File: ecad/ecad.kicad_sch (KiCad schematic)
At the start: 0 parts

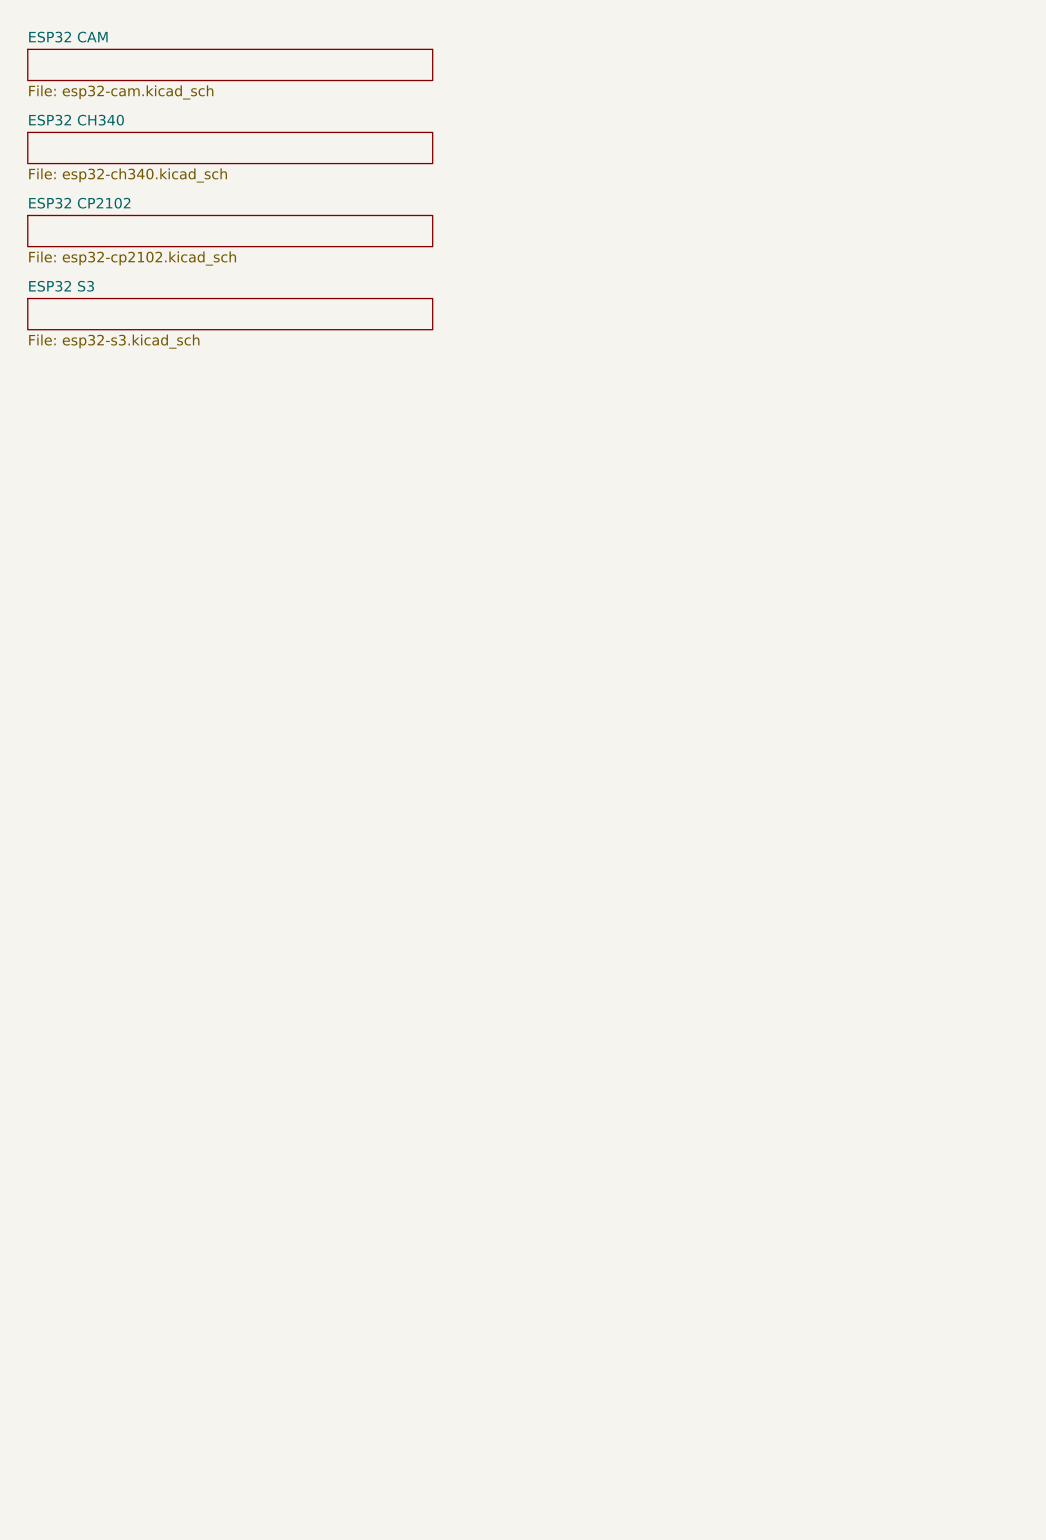
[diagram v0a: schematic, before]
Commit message: feat (ecad): update KiCad project
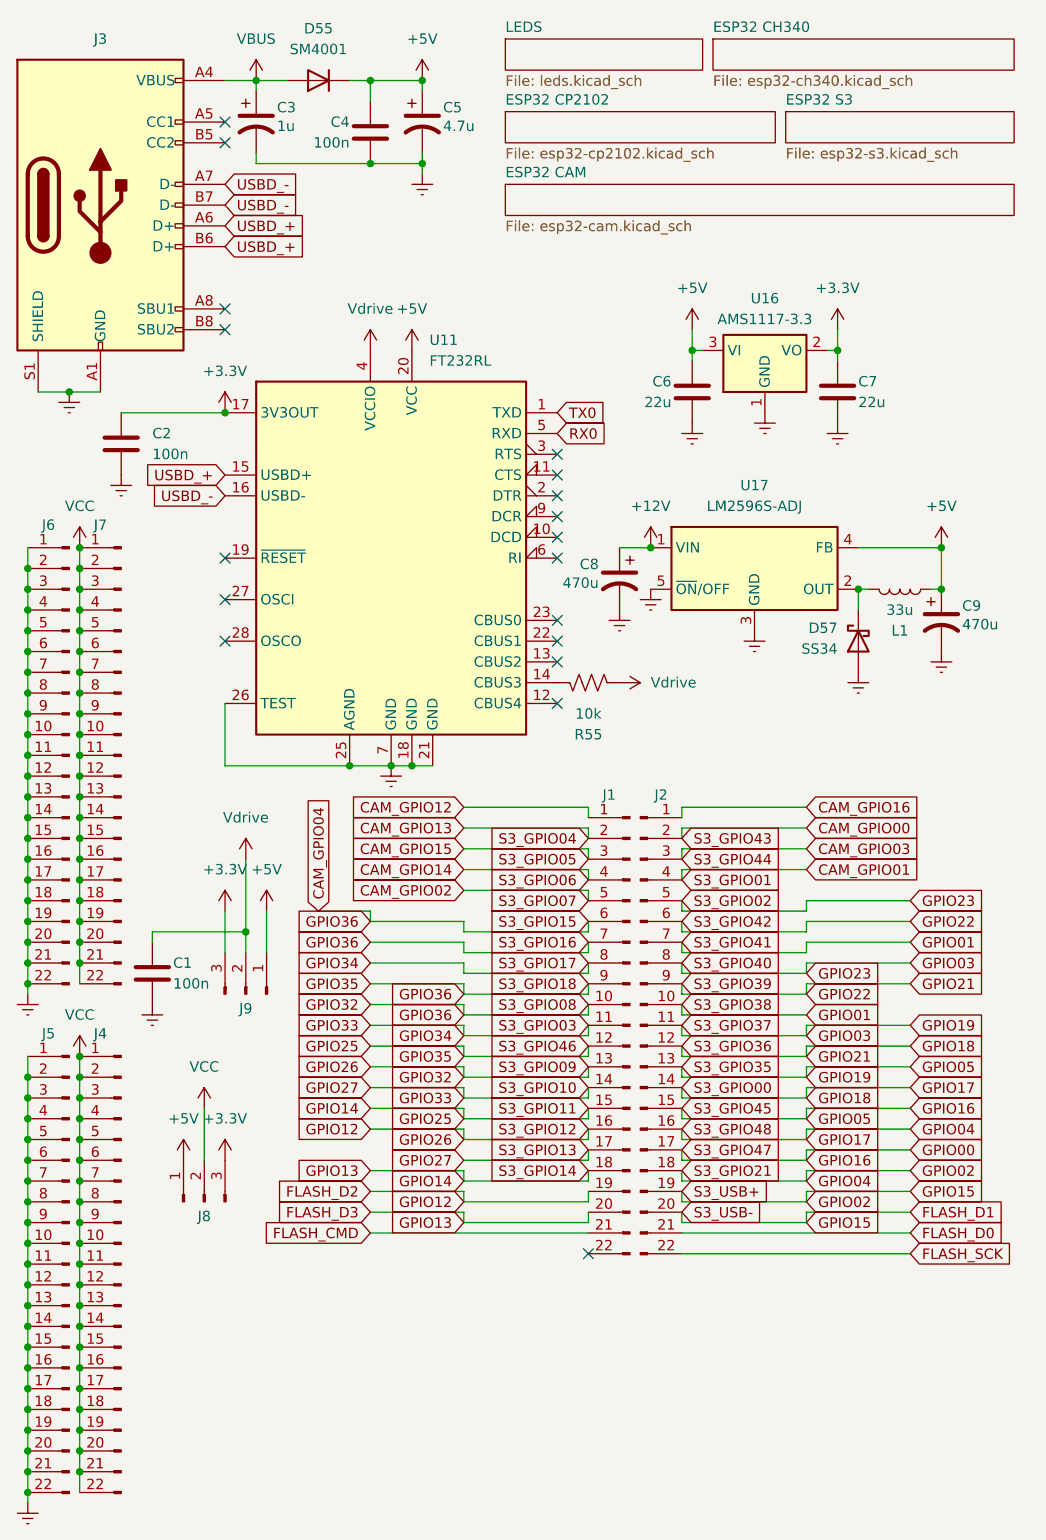
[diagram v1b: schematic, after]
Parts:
- added C1, C2, C4: 100n, Capacitor_SMD:C_0805_2012Metric_Pad1.18x1.45mm_HandSolder, symbol Device:C
- added C3: 1u, Capacitor_SMD:CP_Elec_4x5.4, symbol Device:C_Polarized_US
- added C5: 4.7u, Capacitor_SMD:CP_Elec_4x5.4, symbol Device:C_Polarized_US
- added C6, C7: 22u, Capacitor_SMD:C_0805_2012Metric_Pad1.18x1.45mm_HandSolder, symbol Device:C
- added C8, C9: 470u, Capacitor_SMD:CP_Elec_8x10.5, symbol Device:C_Polarized_US
- added D55: SM4001, Diode_SMD:D_MELF, symbol Diode:SM4001
- added D57: SS34, Diode_SMD:D_SMA, symbol Diode:SS34
- added J1, J2, J4, J5, J6, J7: Conn_01x22_Pin, Connector_PinHeader_2.54mm:PinHeader_1x22_P2.54mm_Vertical, symbol Connector:Conn_01x22_Pin
- added J3: USB_C, Connector_USB:USB_C_Receptacle_Palconn_UTC16-G, symbol Connector:USB_C_Receptacle_USB2.0_16P
- added J8, J9: Conn_01x03_Pin, Connector_PinHeader_2.54mm:PinHeader_1x03_P2.54mm_Vertical, symbol Connector:Conn_01x03_Pin
- added L1: 33u, Inductor_SMD:L_6.3x6.3_H3, symbol Device:L
- added R55: 10k, Resistor_SMD:R_0805_2012Metric_Pad1.20x1.40mm_HandSolder, symbol Device:R_US
- added U11: FT232RL, Package_SO:SSOP-28_5.3x10.2mm_P0.65mm, symbol Interface_USB:FT232RL
- added U16: AMS1117-3.3, Package_TO_SOT_SMD:SOT-223-3_TabPin2, symbol Regulator_Linear:AMS1117-3.3
- added U17: LM2596S-ADJ, Package_TO_SOT_SMD:TO-263-5_TabPin3, symbol Regulator_Switching:LM2596S-ADJ
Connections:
- new net: R55.1, U11.14 (CBUS3)
- new net: D57.1 (K), L1.1, U17.2 (OUT)
- new net +12V: C8.1, U17.1 (VIN)
- new net +3.3V: C2.1, C7.1, J8.3 (Pin_3), J9.3 (Pin_3), U11.17 (3V3OUT), U16.2 (VO)
- new net +5V: C4.1, C5.1, C6.1, C9.1, D55.1 (K), J8.1 (Pin_1), J9.1 (Pin_1), L1.2, U11.20 (VCC), U16.3 (VI), U17.4 (FB)
- new net CAM_GPIO00: J2.2 (Pin_2)
- new net CAM_GPIO01: J2.4 (Pin_4)
- new net CAM_GPIO02: J1.5 (Pin_5)
- new net CAM_GPIO03: J2.3 (Pin_3)
- new net CAM_GPIO04: J1.10 (Pin_10), J1.12 (Pin_12), J1.13 (Pin_13), J1.15 (Pin_15), J1.16 (Pin_16), J1.18 (Pin_18), J1.19 (Pin_19), J1.20 (Pin_20), J1.6 (Pin_6), J1.7 (Pin_7), J1.9 (Pin_9)
- new net CAM_GPIO12: J1.1 (Pin_1)
- new net CAM_GPIO13: J1.2 (Pin_2)
- new net CAM_GPIO14: J1.4 (Pin_4)
- new net CAM_GPIO15: J1.3 (Pin_3)
- new net CAM_GPIO16: J2.1 (Pin_1)
- new net Earth: C1.2, C2.2, C3.2, C4.2, C5.2, C6.2, C7.2, C8.2, C9.2, D57.2 (A), J3.A1 (GND), J3.A12 (GND), J3.B1 (GND), J3.B12 (GND), J3.S1 (SHIELD), J5.1 (Pin_1), J5.10 (Pin_10), J5.11 (Pin_11), J5.12 (Pin_12), J5.13 (Pin_13), J5.14 (Pin_14), J5.15 (Pin_15), J5.16 (Pin_16), J5.17 (Pin_17), J5.18 (Pin_18), J5.19 (Pin_19), J5.2 (Pin_2), J5.20 (Pin_20), J5.21 (Pin_21), J5.22 (Pin_22), J5.3 (Pin_3), J5.4 (Pin_4), J5.5 (Pin_5), J5.6 (Pin_6), J5.7 (Pin_7), J5.8 (Pin_8), J5.9 (Pin_9), J6.1 (Pin_1), J6.10 (Pin_10), J6.11 (Pin_11), J6.12 (Pin_12), J6.13 (Pin_13), J6.14 (Pin_14), J6.15 (Pin_15), J6.16 (Pin_16), J6.17 (Pin_17), J6.18 (Pin_18), J6.19 (Pin_19), J6.2 (Pin_2), J6.20 (Pin_20), J6.21 (Pin_21), J6.22 (Pin_22), J6.3 (Pin_3), J6.4 (Pin_4), J6.5 (Pin_5), J6.6 (Pin_6), J6.7 (Pin_7), J6.8 (Pin_8), J6.9 (Pin_9), U11.18 (GND), U11.21 (GND), U11.25 (AGND), U11.26 (TEST), U11.7 (GND), U16.1 (GND), U17.3 (GND), U17.5 (~{ON}/OFF)
- new net FLASH_CMD: J1.21 (Pin_21)
- new net FLASH_D0: J2.21 (Pin_21)
- new net FLASH_D1: J2.12 (Pin_12), J2.14 (Pin_14), J2.16 (Pin_16), J2.18 (Pin_18), J2.19 (Pin_19), J2.20 (Pin_20), J2.6 (Pin_6), J2.9 (Pin_9)
- new net FLASH_SCK: J2.22 (Pin_22)
- new net GPIO00: J2.11 (Pin_11), J2.13 (Pin_13), J2.15 (Pin_15), J2.17 (Pin_17), J2.5 (Pin_5), J2.8 (Pin_8)
- new net GPIO01: J2.10 (Pin_10), J2.7 (Pin_7)
- new net GPIO27: J1.11 (Pin_11), J1.14 (Pin_14), J1.17 (Pin_17), J1.8 (Pin_8)
- new net RX0: U11.5 (RXD)
- new net TX0: U11.1 (TXD)
- new net USBD_+: J3.A6 (D+), J3.B6 (D+), U11.15 (USBD+)
- new net USBD_-: J3.A7 (D-), J3.B7 (D-), U11.16 (USBD-)
- new net VBUS: C3.1, D55.2 (A), J3.A4 (VBUS), J3.A9 (VBUS), J3.B4 (VBUS), J3.B9 (VBUS)
- new net VCC: J4.1 (Pin_1), J4.10 (Pin_10), J4.11 (Pin_11), J4.12 (Pin_12), J4.13 (Pin_13), J4.14 (Pin_14), J4.15 (Pin_15), J4.16 (Pin_16), J4.17 (Pin_17), J4.18 (Pin_18), J4.19 (Pin_19), J4.2 (Pin_2), J4.20 (Pin_20), J4.21 (Pin_21), J4.22 (Pin_22), J4.3 (Pin_3), J4.4 (Pin_4), J4.5 (Pin_5), J4.6 (Pin_6), J4.7 (Pin_7), J4.8 (Pin_8), J4.9 (Pin_9), J7.1 (Pin_1), J7.10 (Pin_10), J7.11 (Pin_11), J7.12 (Pin_12), J7.13 (Pin_13), J7.14 (Pin_14), J7.15 (Pin_15), J7.16 (Pin_16), J7.17 (Pin_17), J7.18 (Pin_18), J7.19 (Pin_19), J7.2 (Pin_2), J7.20 (Pin_20), J7.21 (Pin_21), J7.22 (Pin_22), J7.3 (Pin_3), J7.4 (Pin_4), J7.5 (Pin_5), J7.6 (Pin_6), J7.7 (Pin_7), J7.8 (Pin_8), J7.9 (Pin_9), J8.2 (Pin_2)
- new net Vdrive: C1.1, J9.2 (Pin_2), R55.2, U11.4 (VCCIO)
- no-connect marks 0 -> 18
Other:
- added sheet LEDS (leds.kicad_sch)
- title: ESP32 AK Shield Schematik drawing -> ESP32 AK Shield Schematik drawing ROOT

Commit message: feat (ecad): update KiCad project
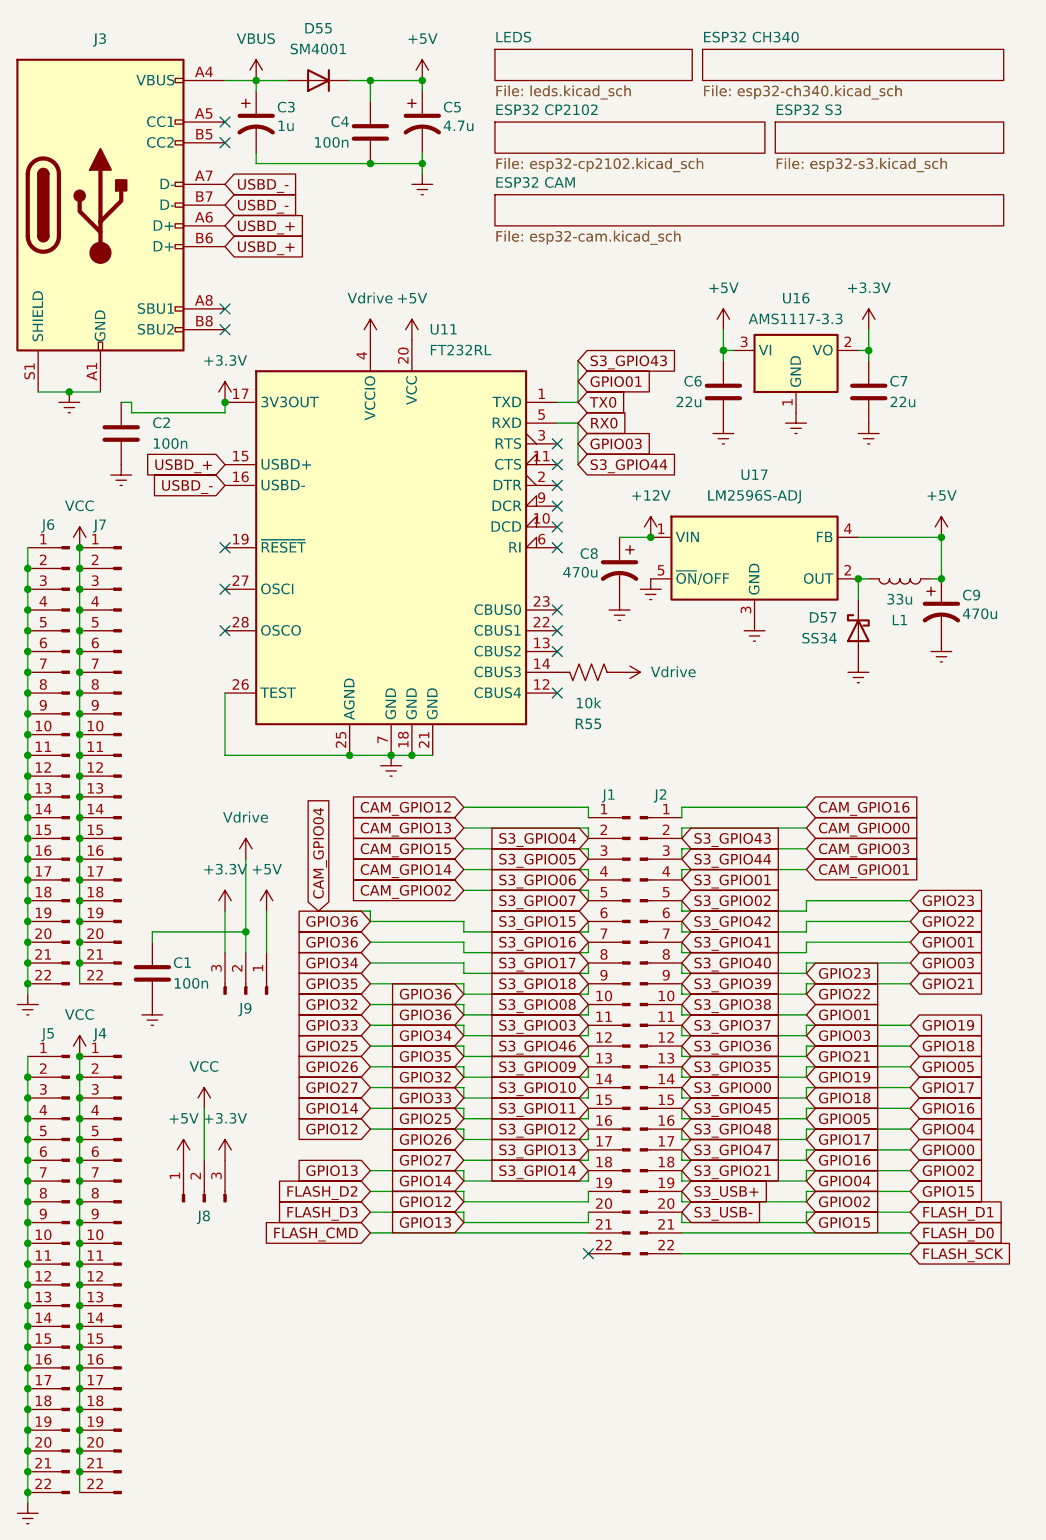
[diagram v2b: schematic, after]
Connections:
- net GPIO00 is gone; now on net CAM_GPIO03: J2.11 (Pin_11), J2.13 (Pin_13), J2.15 (Pin_15), J2.17 (Pin_17), J2.5 (Pin_5), J2.8 (Pin_8)
- net GPIO01 is gone; now on net CAM_GPIO00: J2.10 (Pin_10), J2.7 (Pin_7)
- net RX0 is gone; now on net CAM_GPIO03: U11.5 (RXD)
- net TX0 is gone; now on net CAM_GPIO00: U11.1 (TXD)
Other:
- moved on the sheet: C2, C6, C7, C8, C9, D57, L1, R55, U11, U16, U17
